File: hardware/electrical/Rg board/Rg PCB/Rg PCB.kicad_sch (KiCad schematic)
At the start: 8 parts, among them J1 Conn_01x03, J2 Conn_01x01_Pin

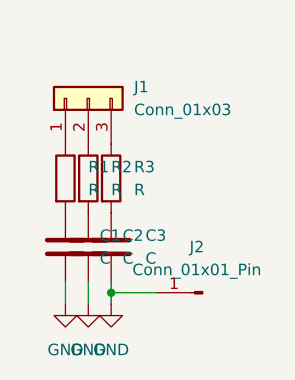
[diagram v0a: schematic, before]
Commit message: update fw readme
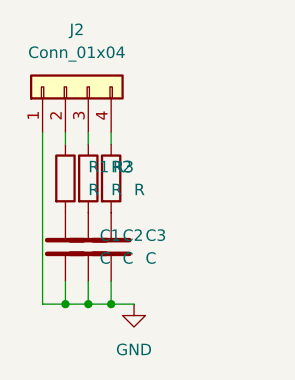
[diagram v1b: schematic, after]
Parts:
- removed J1: Conn_01x03, Connector_PinHeader_2.54mm:PinHeader_1x03_P2.54mm_Vertical, symbol Connector_Generic:Conn_01x03
- removed J2: Conn_01x01_Pin, Connector_PinHeader_2.54mm:PinHeader_1x01_P2.54mm_Vertical, symbol Connector:Conn_01x01_Pin
- added J2: Conn_01x04, Connector_PinHeader_2.54mm:PinHeader_1x04_P2.54mm_Vertical, symbol Connector_Generic:Conn_01x04
- R1, R2, R3: footprint Resistor_THT:R_Axial_DIN0207_L6.3mm_D2.5mm_P10.16mm_Horizontal -> Resistor_THT:R_Axial_DIN0207_L6.3mm_D2.5mm_P7.62mm_Horizontal
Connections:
- net GND: now also J2.1 (Pin_1)
- net at R2.1: now also J2.3 (Pin_3)
- net at R1.1: now also J2.2 (Pin_2)
- net at R3.1: now also J2.4 (Pin_4)
